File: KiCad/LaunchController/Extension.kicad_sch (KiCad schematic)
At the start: 3 parts, among them J7 CONN_STATUS_PANEL, J8 CONN_PANEL_BAORD_2, J9 CONN_PANEL_BAORD_1

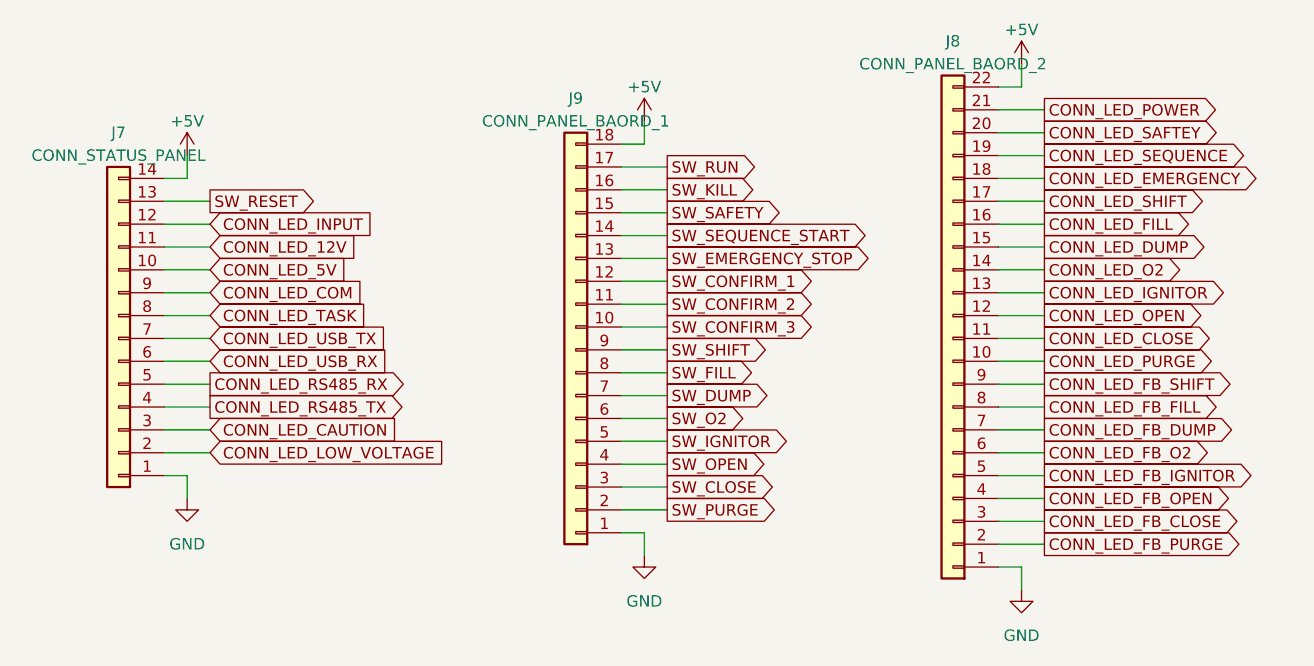
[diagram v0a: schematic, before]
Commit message: ランコンおわり
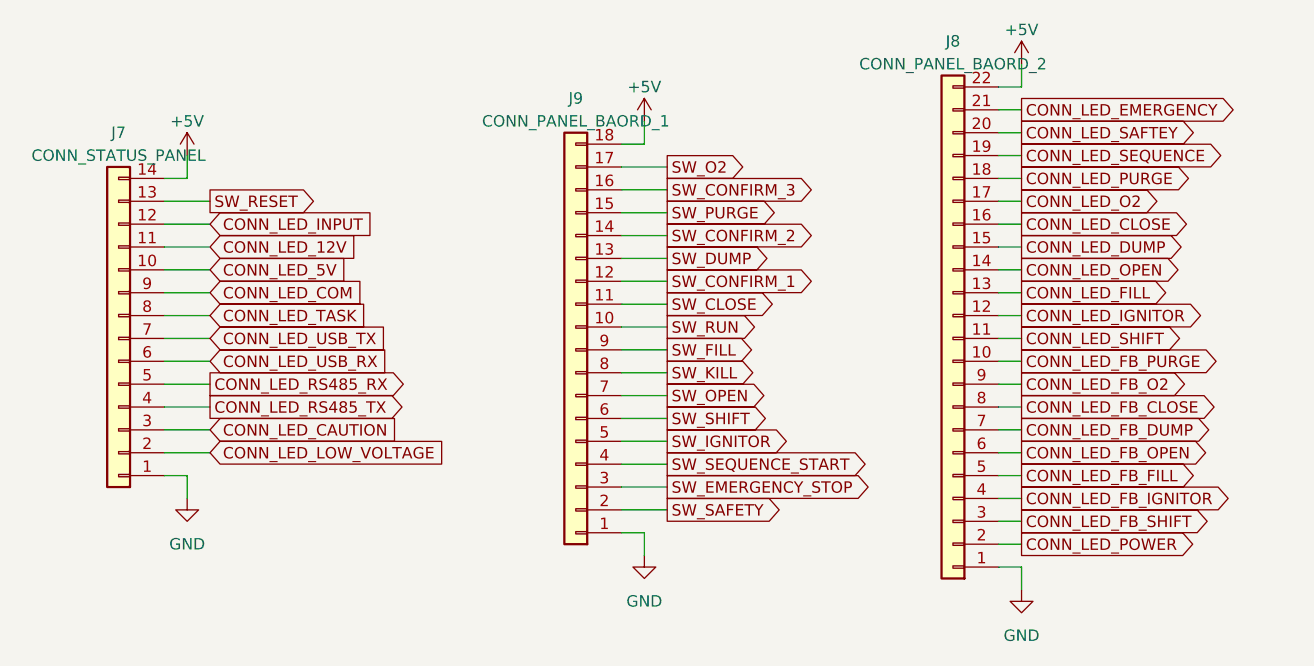
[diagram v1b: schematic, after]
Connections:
- net CONN_LED_CLOSE: now also J8.16 (Pin_16); no longer J8.11 (Pin_11)
- net CONN_LED_EMERGENCY: now also J8.21 (Pin_21); no longer J8.18 (Pin_18)
- net CONN_LED_FB_CLOSE: now also J8.8 (Pin_8); no longer J8.3 (Pin_3)
- net CONN_LED_FB_FILL: now also J8.5 (Pin_5); no longer J8.8 (Pin_8)
- net CONN_LED_FB_IGNITOR: now also J8.4 (Pin_4); no longer J8.5 (Pin_5)
- net CONN_LED_FB_O2: now also J8.9 (Pin_9); no longer J8.6 (Pin_6)
- net CONN_LED_FB_OPEN: now also J8.6 (Pin_6); no longer J8.4 (Pin_4)
- net CONN_LED_FB_PURGE: now also J8.10 (Pin_10); no longer J8.2 (Pin_2)
- net CONN_LED_FB_SHIFT: now also J8.3 (Pin_3); no longer J8.9 (Pin_9)
- net CONN_LED_FILL: now also J8.13 (Pin_13); no longer J8.16 (Pin_16)
- net CONN_LED_IGNITOR: now also J8.12 (Pin_12); no longer J8.13 (Pin_13)
- net CONN_LED_O2: now also J8.17 (Pin_17); no longer J8.14 (Pin_14)
- net CONN_LED_OPEN: now also J8.14 (Pin_14); no longer J8.12 (Pin_12)
- net CONN_LED_POWER: now also J8.2 (Pin_2); no longer J8.21 (Pin_21)
- net CONN_LED_PURGE: now also J8.18 (Pin_18); no longer J8.10 (Pin_10)
- net CONN_LED_SHIFT: now also J8.11 (Pin_11); no longer J8.17 (Pin_17)
- net SW_CLOSE: now also J9.11 (Pin_11); no longer J9.3 (Pin_3)
- net SW_CONFIRM_2: now also J9.14 (Pin_14); no longer J9.11 (Pin_11)
- net SW_CONFIRM_3: now also J9.16 (Pin_16); no longer J9.10 (Pin_10)
- net SW_DUMP: now also J9.13 (Pin_13); no longer J9.7 (Pin_7)
- net SW_EMERGENCY_STOP: now also J9.3 (Pin_3); no longer J9.13 (Pin_13)
- net SW_FILL: now also J9.9 (Pin_9); no longer J9.8 (Pin_8)
- net SW_KILL: now also J9.8 (Pin_8); no longer J9.16 (Pin_16)
- net SW_O2: now also J9.17 (Pin_17); no longer J9.6 (Pin_6)
- net SW_OPEN: now also J9.7 (Pin_7); no longer J9.4 (Pin_4)
- net SW_PURGE: now also J9.15 (Pin_15); no longer J9.2 (Pin_2)
- net SW_RUN: now also J9.10 (Pin_10); no longer J9.17 (Pin_17)
- net SW_SAFETY: now also J9.2 (Pin_2); no longer J9.15 (Pin_15)
- net SW_SEQUENCE_START: now also J9.4 (Pin_4); no longer J9.14 (Pin_14)
- net SW_SHIFT: now also J9.6 (Pin_6); no longer J9.9 (Pin_9)
